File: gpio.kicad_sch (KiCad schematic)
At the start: 16 parts, among them J10 Conn_01x03_Pin, J11 Conn_01x03_Pin, J12 Conn_01x04_Pin, J13 Conn_01x04_Pin, J14 Conn_01x03_Pin, J19 Conn_01x04_Pin, J20 Conn_01x04_Pin, J21 Conn_01x04_Pin, J7 Conn_01x04_Pin, J8 Conn_01x03_Pin, J9 Conn_01x04_Pin, U10 ULC0524P, U11 ULC0524P, U12 ULC0524P, U17 ULC0524P, U9 ULC0524P

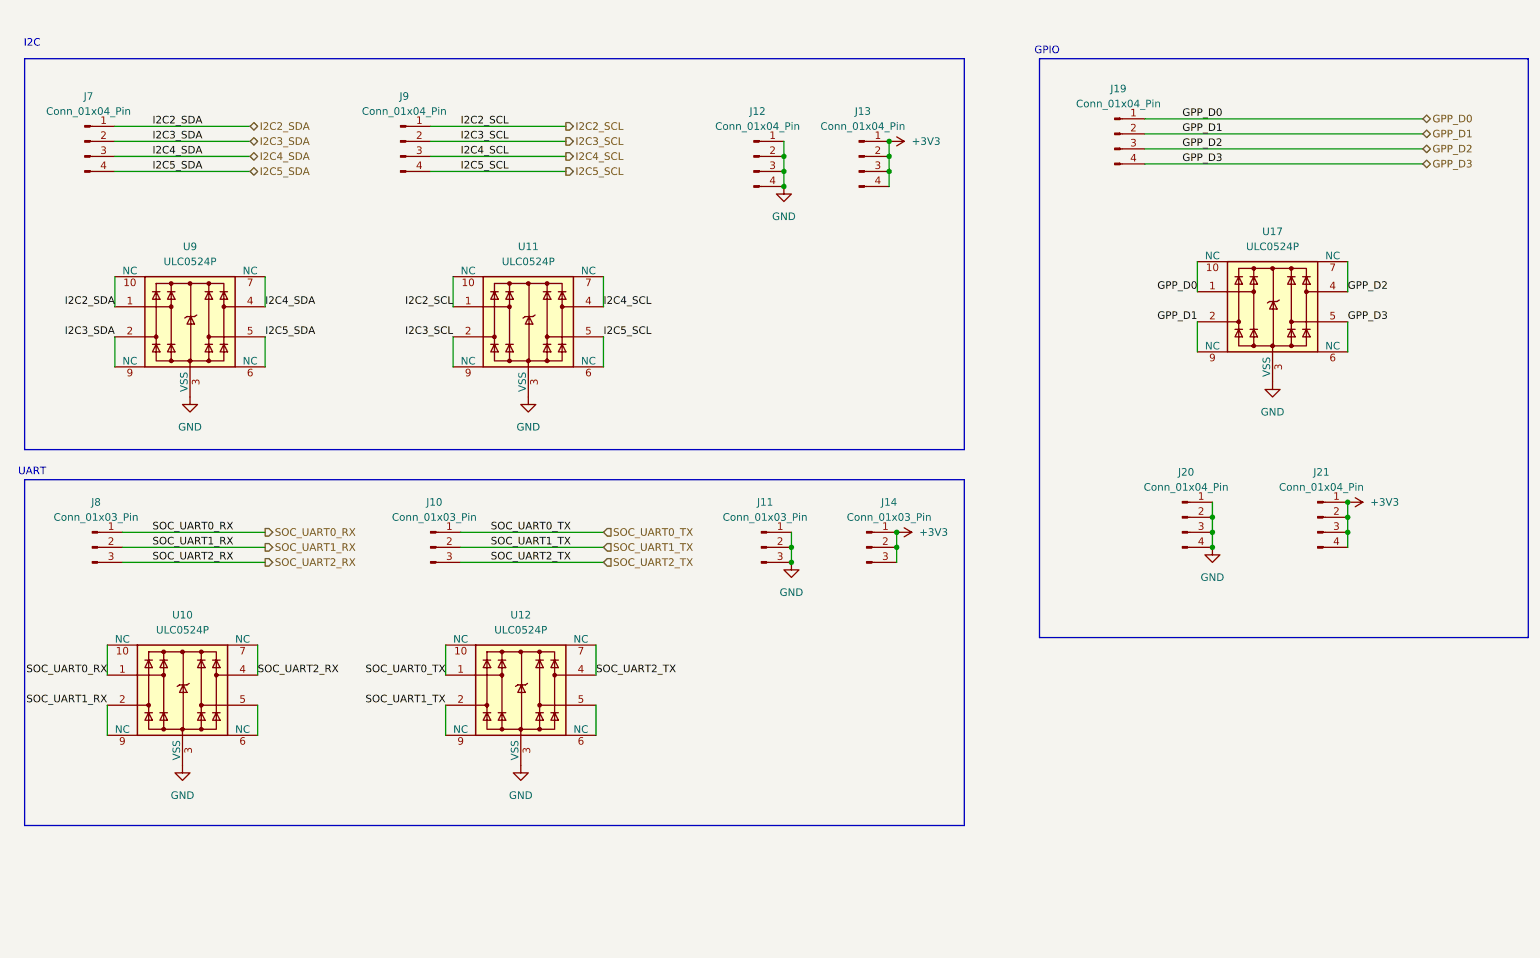
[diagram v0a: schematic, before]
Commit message: added reference design and finished routing
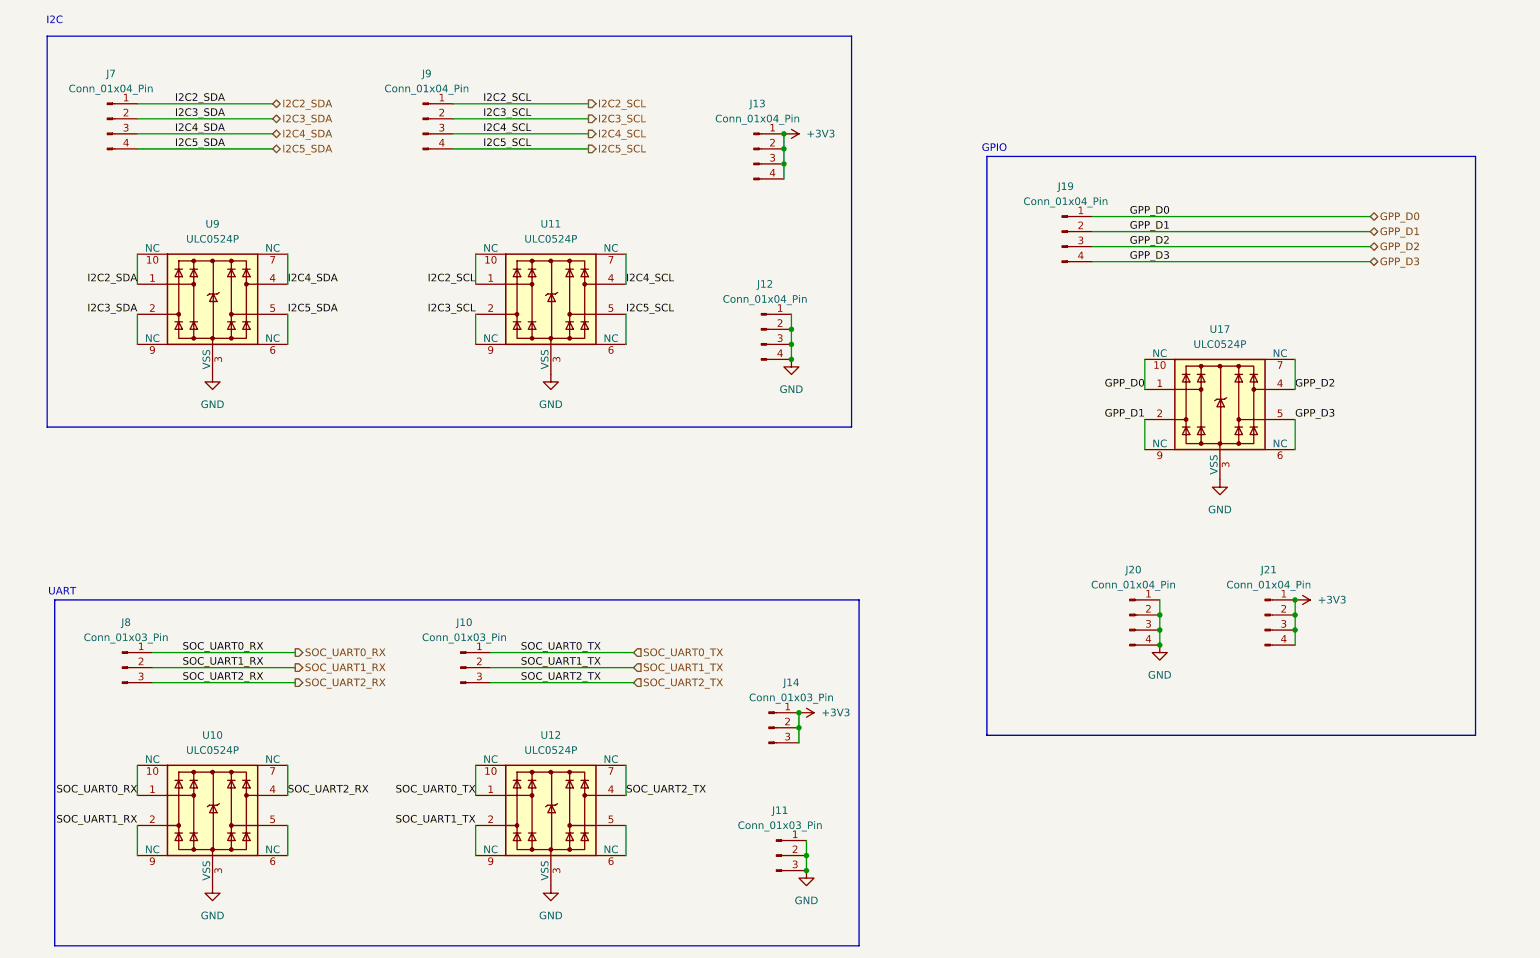
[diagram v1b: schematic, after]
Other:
- moved on the sheet: J10, J11, J12, J13, J14, J19, J20, J21, J7, J8, J9, U10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
